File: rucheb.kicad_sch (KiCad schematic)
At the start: 24 parts, among them IC1 CN3791, J1 Conn_01x02, Q1 AO3401A, U7 1043

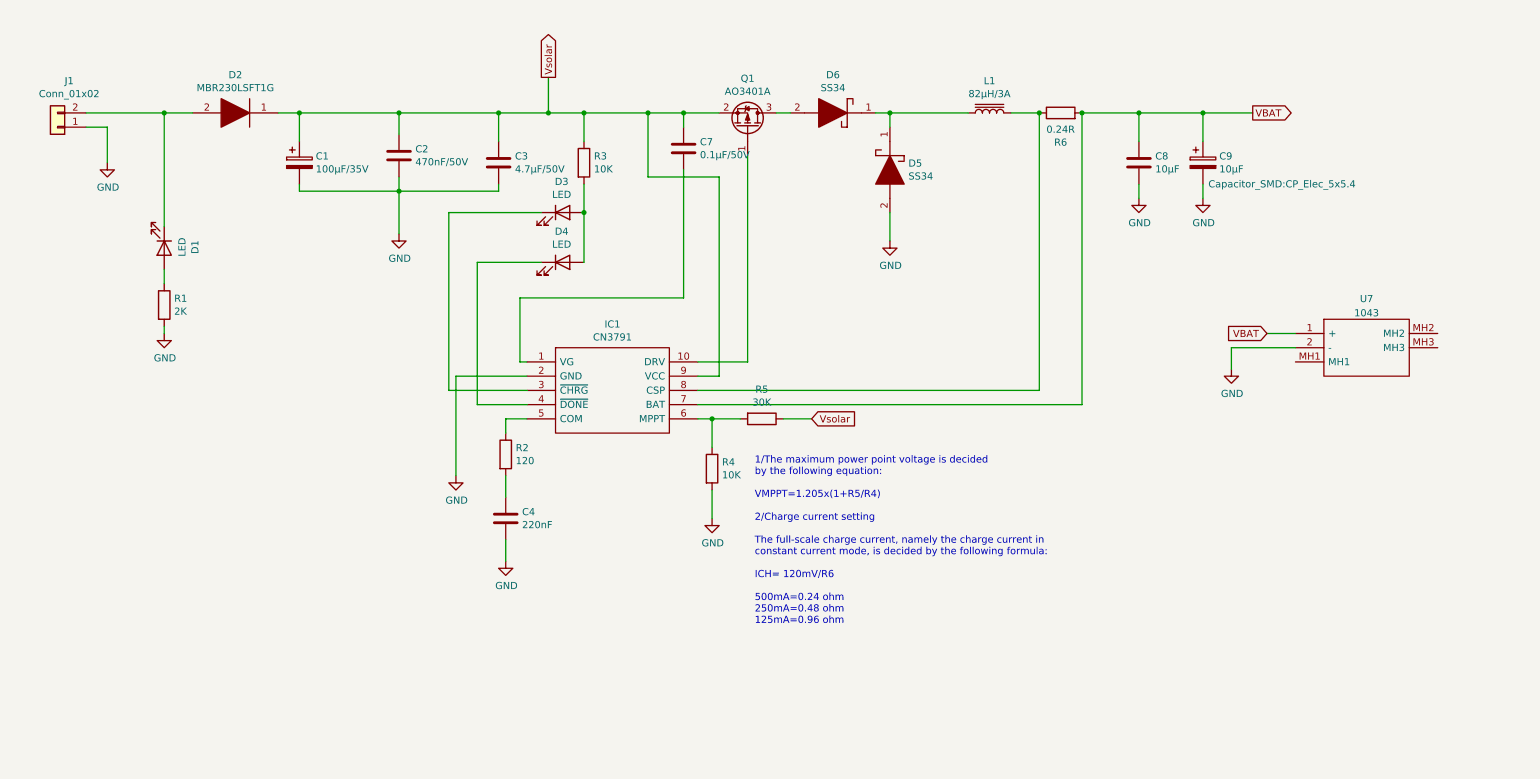
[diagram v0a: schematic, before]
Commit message: update
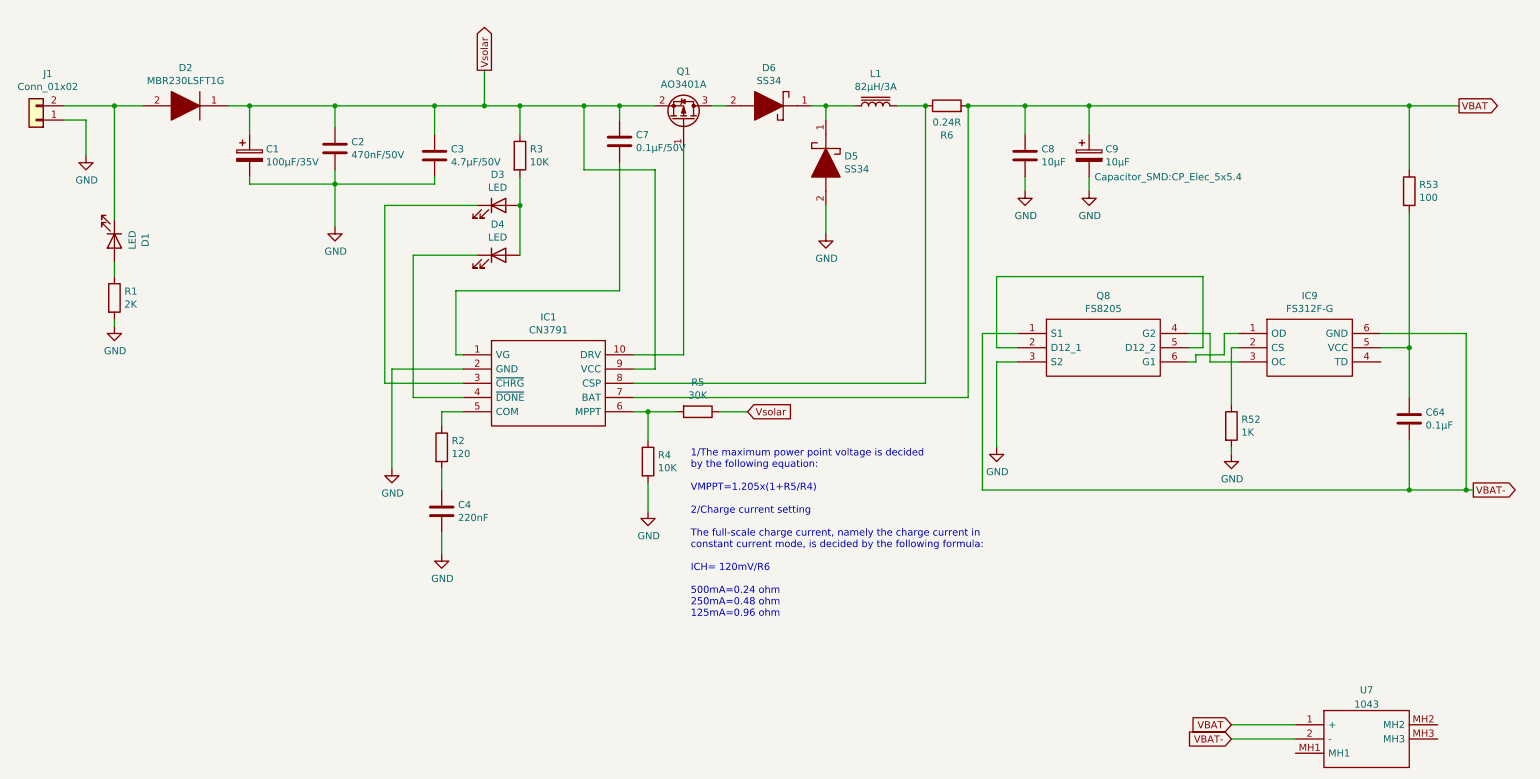
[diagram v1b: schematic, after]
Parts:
- added C64: 0.1µF, Capacitor_SMD:C_0603_1608Metric, symbol Device:C
- added IC9: FS312F-G, Empreintes:SOT95P280X145-6N, symbol FS312F-G:FS312F-G
- added Q8: FS8205, Empreintes:FS8205, symbol FS8205:FS8205
- added R52: 1K, Resistor_SMD:R_0603_1608Metric, symbol Device:R
- added R53: 100, Resistor_SMD:R_0603_1608Metric, symbol Device:R
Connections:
- net GND: now also Q8.3 (S2), R52.2; no longer U7.2 (-)
- net VBAT: now also R53.1
- new net: IC9.2 (CS), R52.1
- new net: C64.1, IC9.5 (VCC), R53.2
- new net: Q8.2 (D12_1), Q8.5 (D12_2)
- new net: IC9.3 (OC), Q8.4 (G2)
- new net: IC9.1 (OD), Q8.6 (G1)
- new net VBAT-: C64.2, IC9.6 (GND), Q8.1 (S1), U7.2 (-)
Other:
- moved on the sheet: C1, C2, C3, C4, C7, C8, C9, D1, D2, D3, D4, D5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
